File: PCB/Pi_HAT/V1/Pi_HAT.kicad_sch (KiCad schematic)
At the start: 10 parts, among them J1 MPU9250, J2 Pi_GPIO, J3 Display

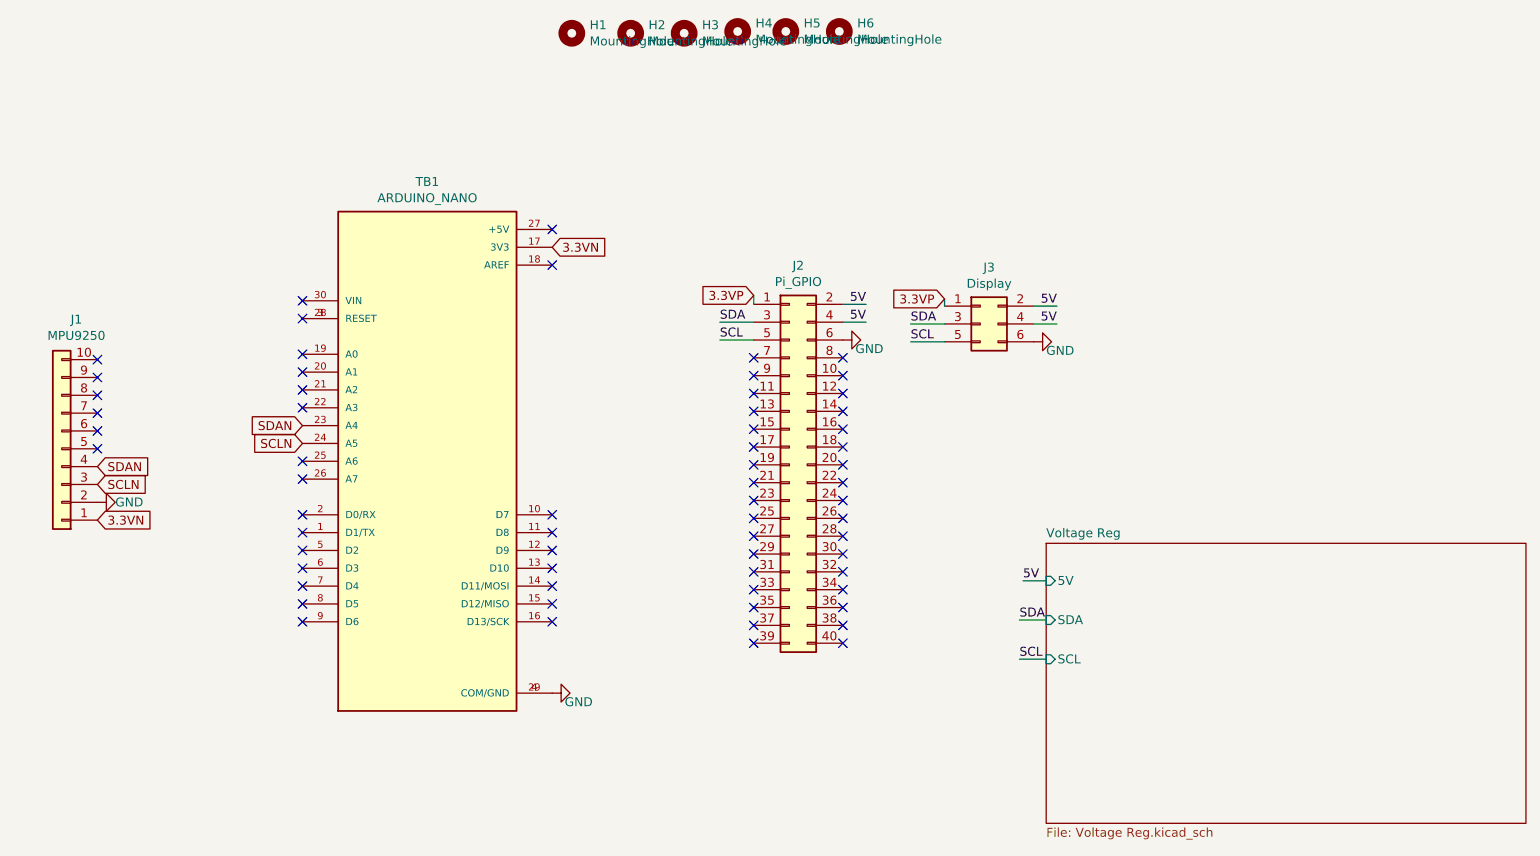
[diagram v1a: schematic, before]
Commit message: Updated V1 Pi Hat
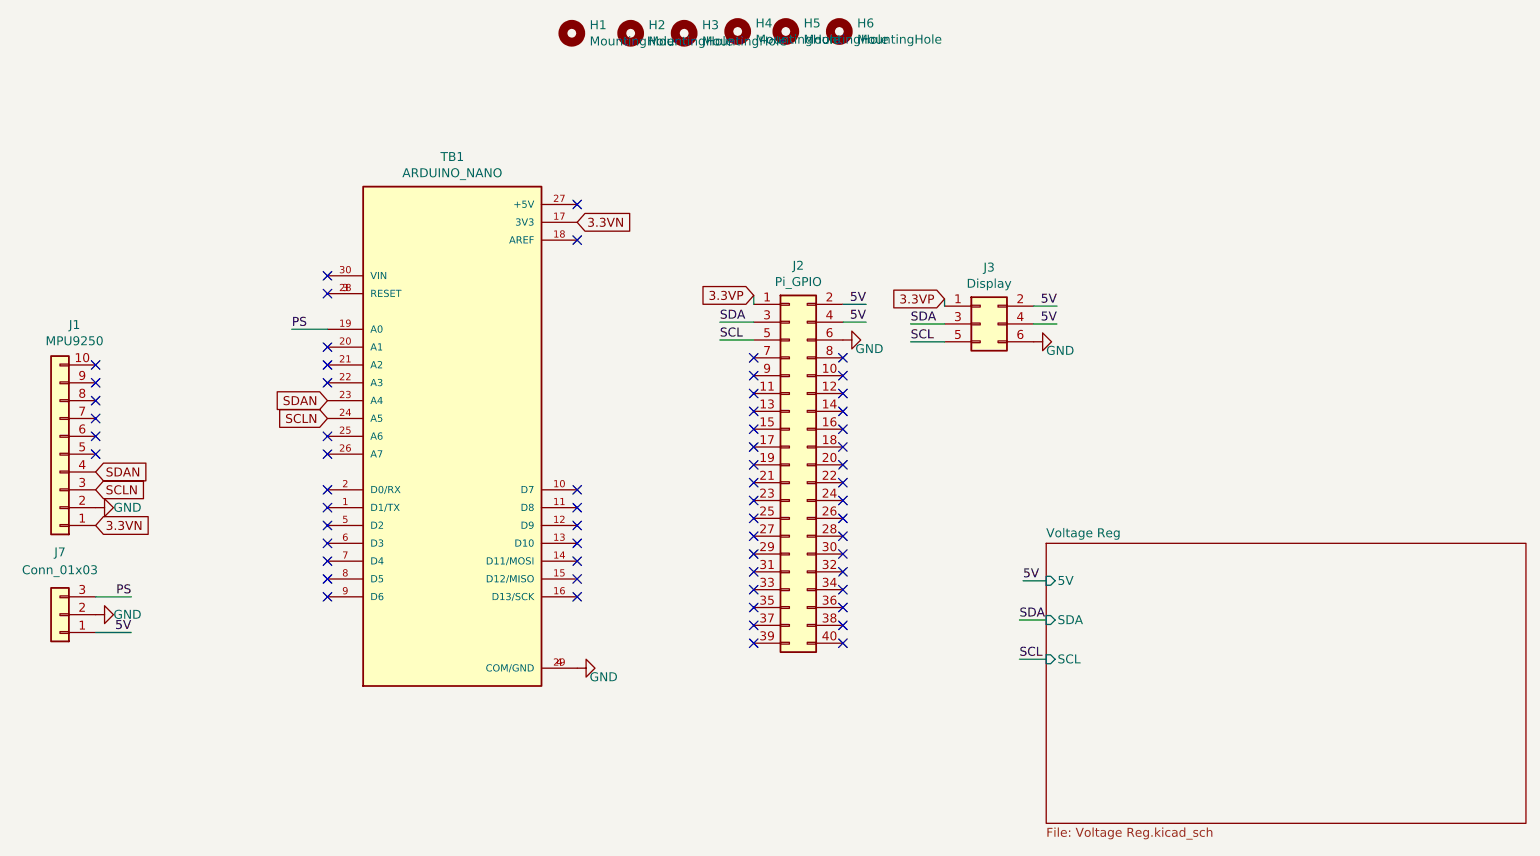
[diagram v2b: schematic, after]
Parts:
- added J7: Conn_01x03, Connector_PinHeader_2.54mm:PinHeader_1x03_P2.54mm_Vertical, symbol Connector_Generic:Conn_01x03
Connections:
- net 5V: now also J7.1 (Pin_1)
- net GND: now also J7.2 (Pin_2)
- net PS: now reaches TB1.19 (A0)
- net PS: now also J7.3 (Pin_3)
- no-connect marks 64 -> 63
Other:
- moved on the sheet: J1, TB1

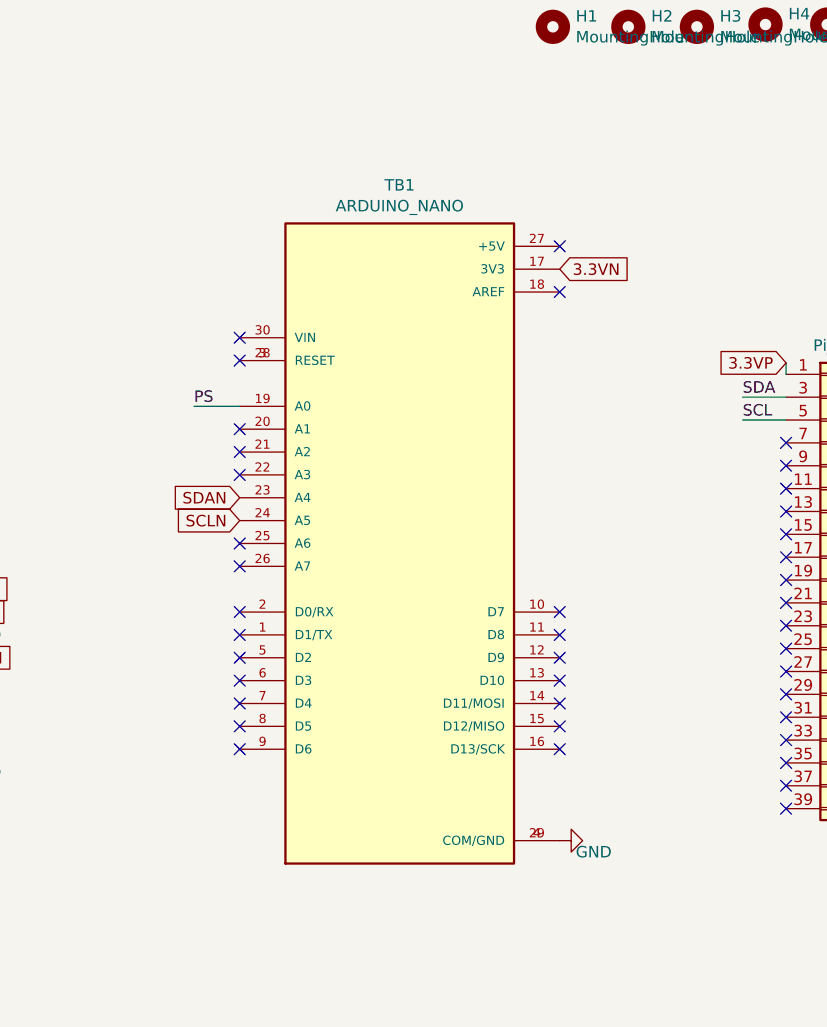
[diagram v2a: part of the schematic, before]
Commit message: Finished V1
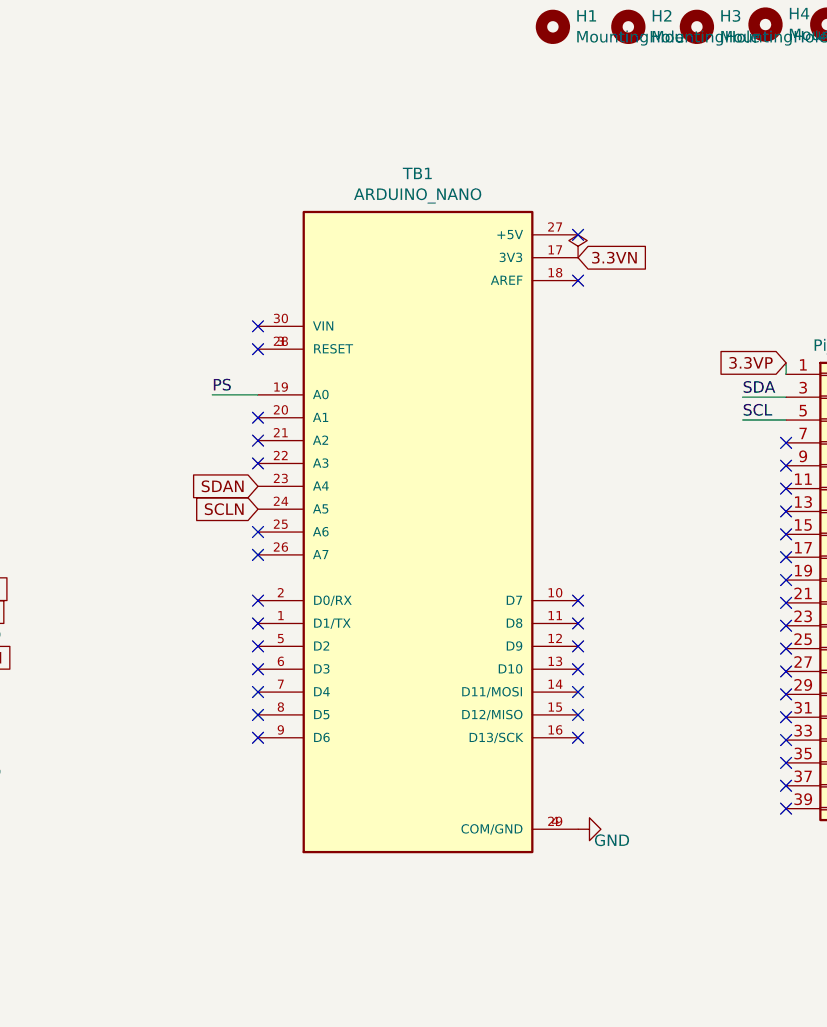
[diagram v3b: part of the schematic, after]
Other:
- moved on the sheet: TB1
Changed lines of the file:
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@@
   (paper "A4")
   (no_connect (at 177.546 95.504))
-  (no_connect (at 104.14 111.76))
+  (no_connect (at 106.172 110.49))
   (no_connect (at 164.846 98.044))
   (no_connect (at 177.546 87.884))
   (no_connect (at 177.546 90.424))
-  (no_connect (at 104.14 88.9))
+  (no_connect (at 106.172 87.63))
   (no_connect (at 177.546 118.364))
-  (no_connect (at 139.7 104.14))
+  (no_connect (at 141.732 102.87))
   (no_connect (at 164.846 110.744))
   (no_connect (at 177.546 80.264))
   (no_connect (at 177.546 77.724))
-  (no_connect (at 139.7 106.68))
-  (no_connect (at 104.14 96.52))
+  (no_connect (at 141.732 105.41))
+  (no_connect (at 106.172 95.25))
   (no_connect (at 164.846 103.124))
   (no_connect (at 71.12 88.9))
   (no_connect (at 177.546 115.824))
   (no_connect (at 177.546 110.744))
-  (no_connect (at 139.7 101.6))
-  (no_connect (at 104.14 109.22))
+  (no_connect (at 141.732 100.33))
+  (no_connect (at 106.172 107.95))
   (no_connect (at 164.846 100.584))
   (no_connect (at 164.846 108.204))
@@
   (no_connect (at 177.546 105.664))
   (no_connect (at 177.546 85.344))
-  (no_connect (at 104.14 76.2))
+  (no_connect (at 106.172 74.93))
   (no_connect (at 177.546 82.804))
   (no_connect (at 71.12 81.28))
   (no_connect (at 71.12 91.44))
-  (no_connect (at 104.14 66.04))
+  (no_connect (at 106.172 64.77))
   (no_connect (at 164.846 105.664))
   (no_connect (at 177.546 98.044))
-  (no_connect (at 139.7 96.52))
+  (no_connect (at 141.732 95.25))
   (no_connect (at 177.546 100.584))
-  (no_connect (at 139.7 55.88))
-  (no_connect (at 104.14 81.28))
-  (no_connect (at 104.14 101.6))
-  (no_connect (at 104.14 104.14))
+  (no_connect (at 141.732 54.61))
+  (no_connect (at 106.172 80.01))
+  (no_connect (at 106.172 100.33))
+  (no_connect (at 106.172 102.87))
   (no_connect (at 164.846 95.504))
   (no_connect (at 177.546 108.204))
-  (no_connect (at 139.7 99.06))
+  (no_connect (at 141.732 97.79))
   (no_connect (at 71.12 83.82))
   (no_connect (at 164.846 90.424))
-  (no_connect (at 139.7 109.22))
+  (no_connect (at 141.732 107.95))
   (no_connect (at 164.846 115.824))
   (no_connect (at 177.546 92.964))
-  (no_connect (at 139.7 60.96))
+  (no_connect (at 141.732 59.69))
   (no_connect (at 164.846 77.724))
   (no_connect (at 71.12 78.74))
@@
   (no_connect (at 164.846 118.364))
   (no_connect (at 164.846 82.804))
-  (no_connect (at 104.14 99.06))
-  (no_connect (at 104.14 91.44))
-  (no_connect (at 139.7 111.76))
-  (no_connect (at 104.14 68.58))
+  (no_connect (at 106.172 97.79))
+  (no_connect (at 106.172 90.17))
+  (no_connect (at 141.732 110.49))
+  (no_connect (at 106.172 67.31))
   (no_connect (at 177.546 113.284))
-  (no_connect (at 104.14 78.74))
-  (no_connect (at 104.14 106.68))
+  (no_connect (at 106.172 77.47))
+  (no_connect (at 106.172 105.41))
   (no_connect (at 164.846 92.964))
   (no_connect (at 164.846 113.284))
   (no_connect (at 164.846 85.344))
-  (wire (pts (xy 104.14 73.66) (xy 99.06 73.66))
+  (wire (pts (xy 106.172 72.39) (xy 101.092 72.39))
     (stroke (width 0) (type default) (color 0 0 0 0))
   )
@@
     (effects (font (size 1.27 1.27)) (justify right bottom))
   )
-  (label "PS" (at 99.06 73.66 0)
+  (label "PS" (at 101.092 72.39 0)
     (effects (font (size 1.27 1.27)) (justify left bottom))
   )
@@
     (effects (font (size 1.27 1.27)) (justify right bottom))
   )
-  (global_label "3.3VN" (shape input) (at 139.7 58.42 0) (fields_autoplaced)
+  (global_label "3.3VN" (shape input) (at 141.732 57.15 0) (fields_autoplaced)
     (effects (font (size 1.27 1.27)) (justify left))
-    (property "Intersheet References" "${INTERSHEET_REFS}" (id 0) (at 3.556 -3.556 0)
+    (property "Intersheet References" "${INTERSHEET_REFS}" (id 0) (at 5.588 -4.826 0)
       (effects (font (size 1.27 1.27)) hide)
     )
@@
     )
   )
-  (global_label "SCLN" (shape input) (at 104.14 86.36 180) (fields_autoplaced)
+  (global_label "SCLN" (shape input) (at 106.172 85.09 180) (fields_autoplaced)
     (effects (font (size 1.27 1.27)) (justify right))
-    (property "Intersheet References" "${INTERSHEET_REFS}" (id 0) (at 3.556 -3.556 0)
-      (effects (font (size 1.27 1.27)) hide)
-    )
-  )
-  (global_label "SDAN" (shape input) (at 104.14 83.82 180) (fields_autoplaced)
+    (property "Intersheet References" "${INTERSHEET_REFS}" (id 0) (at 5.588 -4.826 0)
+      (effects (font (size 1.27 1.27)) hide)
+    )
+  )
+  (global_label "SDAN" (shape input) (at 106.172 82.55 180) (fields_autoplaced)
     (effects (font (size 1.27 1.27)) (justify right))
-    (property "Intersheet References" "${INTERSHEET_REFS}" (id 0) (at 3.556 -3.556 0)
+    (property "Intersheet References" "${INTERSHEET_REFS}" (id 0) (at 5.588 -4.826 0)
       (effects (font (size 1.27 1.27)) hide)
     )
@@
     )
   )
-  (symbol (lib_id "ARDUINO_NANO:ARDUINO_NANO") (at 121.92 88.9 0) (unit 1)
-    (in_bom yes) (on_board yes)
-    (property "Reference" "TB1" (id 0) (at 121.92 49.0982 0))
-    (property "Value" "ARDUINO_NANO" (id 1) (at 121.92 51.4096 0))
-    (property "Footprint" ".pretty:SHIELD_ARDUINO_NANO" (id 2) (at 121.92 88.9 0)
+  (symbol (lib_id "ARDUINO_NANO:ARDUINO_NANO") (at 123.952 87.63 0) (unit 1)
+    (in_bom yes) (on_board yes)
+    (property "Reference" "TB1" (id 0) (at 123.952 47.8282 0))
+    (property "Value" "ARDUINO_NANO" (id 1) (at 123.952 50.1396 0))
+    (property "Footprint" ".pretty:SHIELD_ARDUINO_NANO" (id 2) (at 123.952 87.63 0)
       (effects (font (size 1.27 1.27)) (justify left bottom) hide)
     )
-    (property "Datasheet" "" (id 3) (at 121.92 88.9 0)
+    (property "Datasheet" "" (id 3) (at 123.952 87.63 0)
       (effects (font (size 1.27 1.27)) (justify left bottom) hide)
     )
@@
     (pin "1")
   )
-  (symbol (lib_id "power:GND") (at 139.7 121.92 90) (unit 1)
-    (in_bom yes) (on_board yes)
-    (property "Reference" "#PWR0109" (id 0) (at 146.05 121.92 0)
-      (effects (font (size 1.27 1.27)) hide)
-    )
-    (property "Value" "GND" (id 1) (at 141.478 123.19 90)
+  (symbol (lib_id "power:GND") (at 141.732 120.65 90) (unit 1)
+    (in_bom yes) (on_board yes)
+    (property "Reference" "#PWR0109" (id 0) (at 148.082 120.65 0)
+      (effects (font (size 1.27 1.27)) hide)
+    )
+    (property "Value" "GND" (id 1) (at 143.51 121.92 90)
       (effects (font (size 1.27 1.27)) (justify right))
     )
-    (property "Footprint" "" (id 2) (at 139.7 121.92 0)
-      (effects (font (size 1.27 1.27)) hide)
-    )
-    (property "Datasheet" "" (id 3) (at 139.7 121.92 0)
+    (property "Footprint" "" (id 2) (at 141.732 120.65 0)
+      (effects (font (size 1.27 1.27)) hide)
+    )
+    (property "Datasheet" "" (id 3) (at 141.732 120.65 0)
       (effects (font (size 1.27 1.27)) hide)
     )
@@
     )
     (property "Datasheet" "" (id 3) (at 71.12 114.3 0)
+      (effects (font (size 1.27 1.27)) hide)
+    )
+    (pin "1")
+  )
+  (symbol (lib_id "power:PWR_FLAG") (at 141.732 57.15 0) (unit 1)
+    (in_bom yes) (on_board yes) (fields_autoplaced)
+    (property "Reference" "#FLG0103" (id 0) (at 141.732 55.245 0)
+      (effects (font (size 1.27 1.27)) hide)
+    )
+    (property "Value" "" (id 1) (at 141.732 52.07 0))
+    (property "Footprint" "" (id 2) (at 141.732 57.15 0)
+      (effects (font (size 1.27 1.27)) hide)
+    )
+    (property "Datasheet" "~" (id 3) (at 141.732 57.15 0)
       (effects (font (size 1.27 1.27)) hide)
     )
@@
       (reference "#FLG0102") (unit 1) (value "PWR_FLAG") (footprint "")
     )
+    (path "/280b868d-51ec-4b79-8c2e-2e1621fd18c8"
+      (reference "#FLG0103") (unit 1) (value "PWR_FLAG") (footprint "")
+    )
     (path "/00000000-0000-0000-0000-00006251fa46/00000000-0000-0000-0000-000062525296"
